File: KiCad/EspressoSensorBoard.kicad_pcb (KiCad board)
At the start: 2 copper layers, 130 x 24 mm, 16 parts, among them IC1 FDC1004DGSR, J1 GRAPHIC DISPLAY IPS - 1.69", J2 MAX31855 (Temperature), J3 Screw_Terminal_01x02, J5 Pressure_Sensor, J7 Arduino_Nano_v3_Left, J8 Arduino_Nano_v3_Right, J9 Water_Level_Electrodes

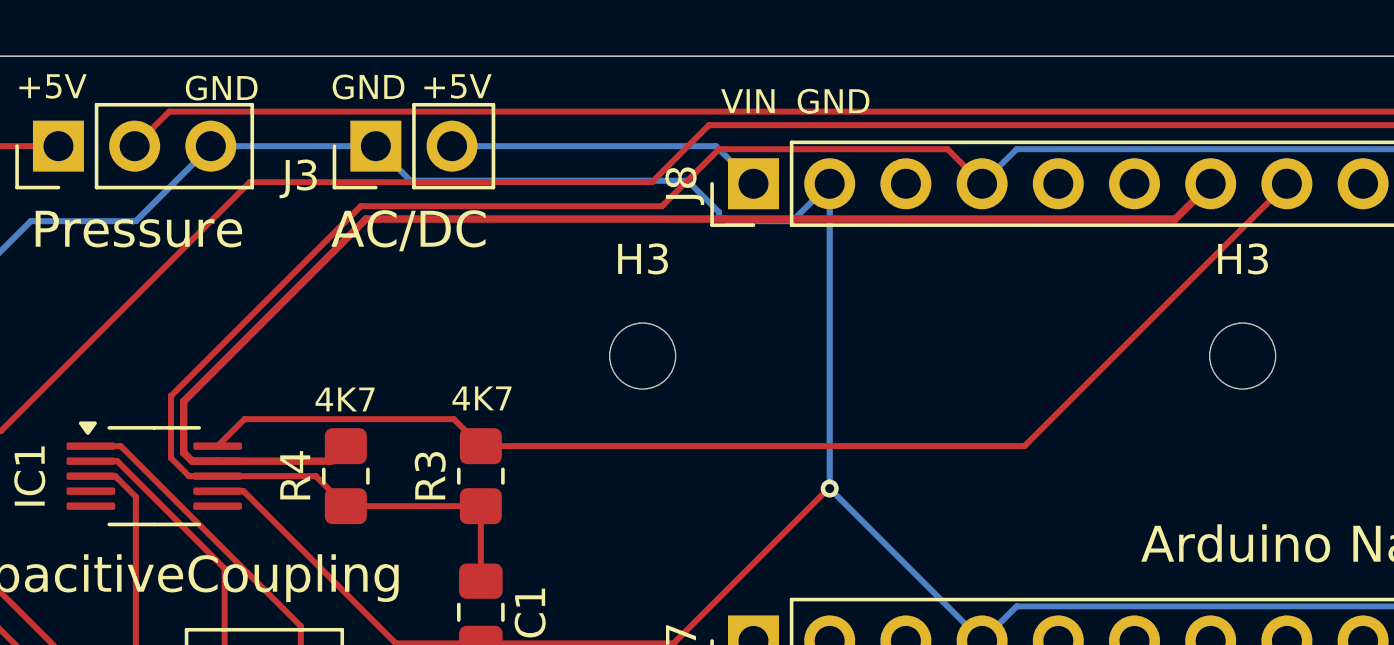
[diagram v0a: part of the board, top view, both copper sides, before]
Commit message: Minor modifs on the Kicad PCD
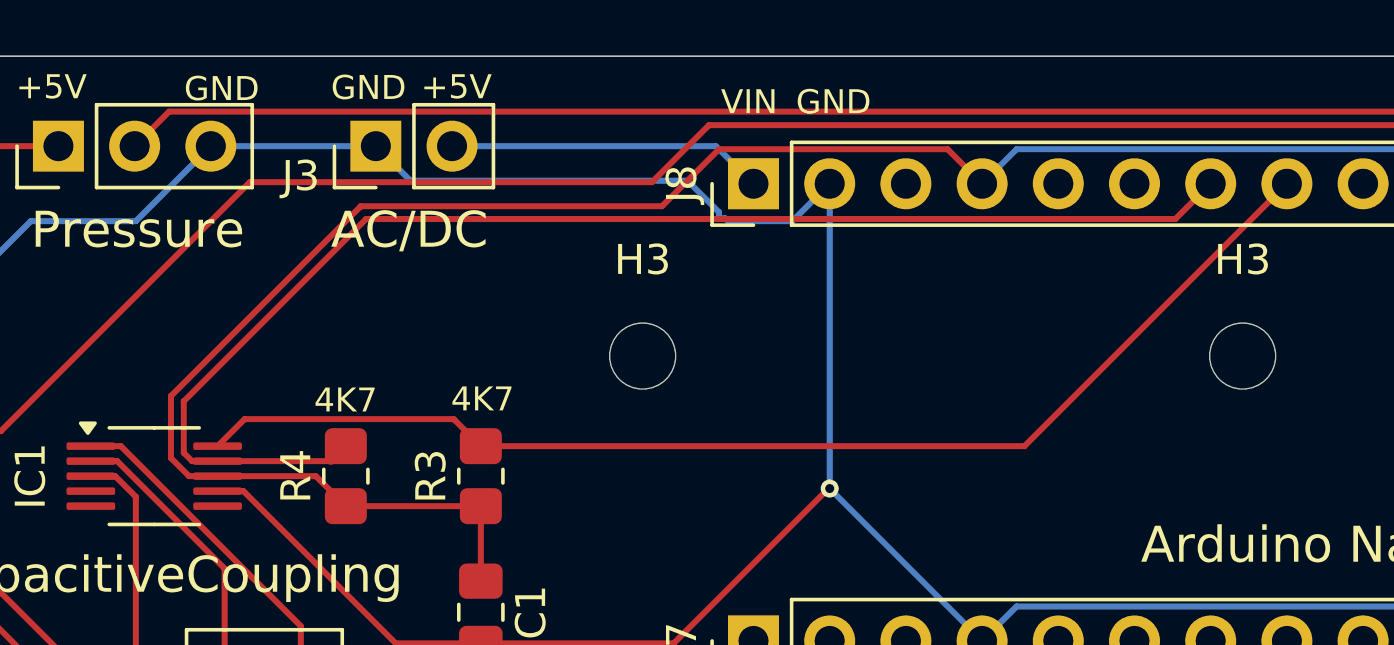
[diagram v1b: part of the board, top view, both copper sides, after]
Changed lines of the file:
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@@
 		(start 112.875488 69.5)
 		(end 113.725 69.5)
-		(width 0.25)
+		(width 0.2)
 		(layer "F.Cu")
 		(net 34)
@@
 		(start 145.652288 61.429084)
 		(end 118.67337 61.429084)
-		(width 0.25)
+		(width 0.2)
 		(layer "F.Cu")
 		(net 34)
@@
 		(start 146.828288 60.253084)
 		(end 145.652288 61.429084)
-		(width 0.25)
+		(width 0.2)
 		(layer "F.Cu")
 		(net 34)
@@
 		(start 112.5965 67.505954)
 		(end 112.5965 69.221012)
-		(width 0.25)
+		(width 0.2)
 		(layer "F.Cu")
 		(net 34)
@@
 		(start 117.5 69.5)
 		(end 113.725 69.5)
-		(width 0.25)
+		(width 0.2)
 		(layer "F.Cu")
 		(net 34)
@@
 		(start 118.67337 61.429084)
 		(end 112.5965 67.505954)
-		(width 0.25)
+		(width 0.2)
 		(layer "F.Cu")
 		(net 34)
@@
 		(start 112.5965 69.221012)
 		(end 112.875488 69.5)
-		(width 0.25)
+		(width 0.2)
 		(layer "F.Cu")
 		(net 34)
